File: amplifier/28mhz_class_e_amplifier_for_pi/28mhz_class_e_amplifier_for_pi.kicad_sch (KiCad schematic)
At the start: 23 parts, among them J1 Conn_Coaxial_Small, J2 694106301002, M1 RD16HHF1, U1 LT1818

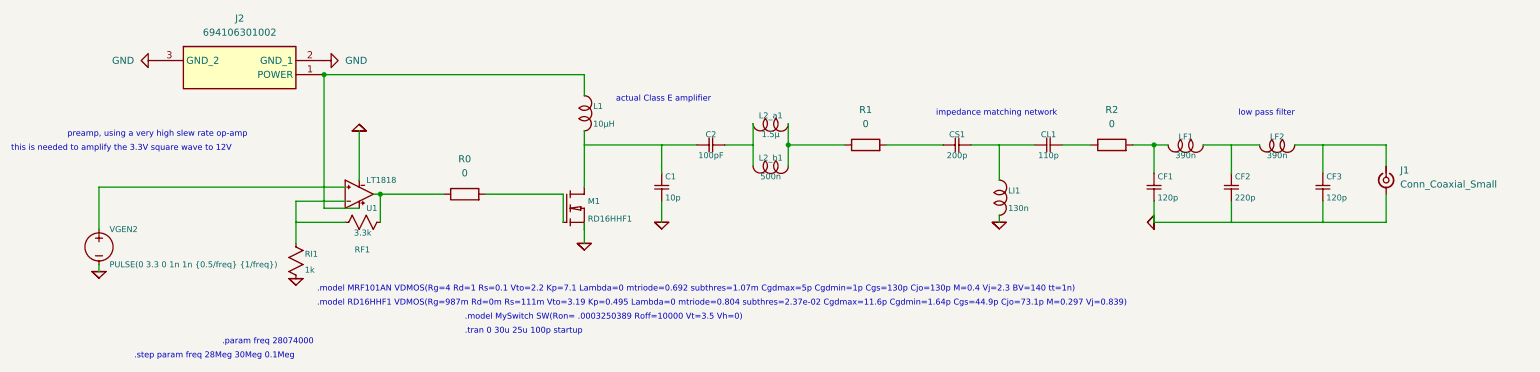
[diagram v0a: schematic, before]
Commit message: Everything except routing done
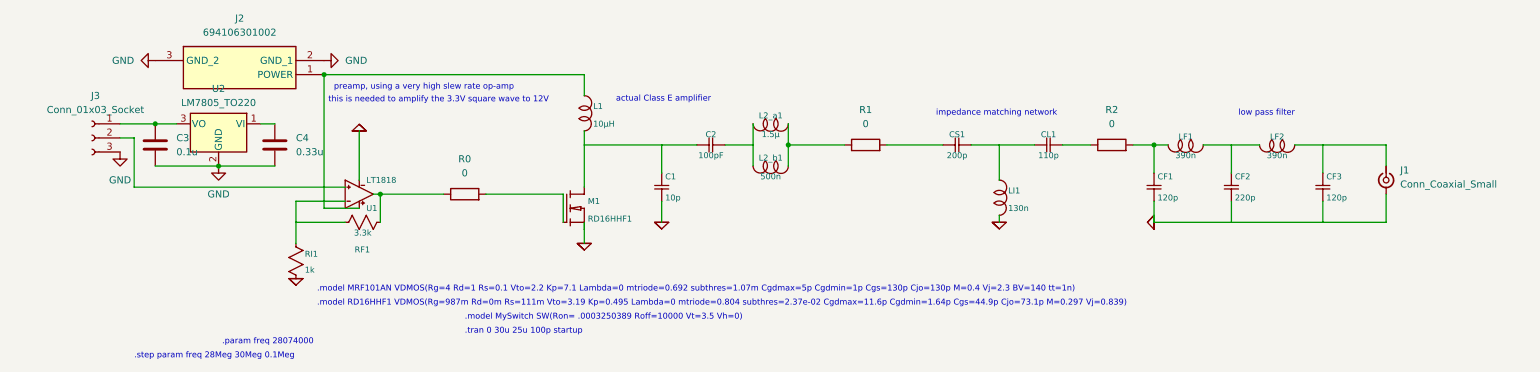
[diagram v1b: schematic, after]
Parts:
- removed VGEN2: PULSE(0 3.3 0 1n 1n {0.5/freq} {1/freq}), Connector_PinHeader_2.54mm:PinHeader_1x02_P2.54mm_Vertical, symbol ltspice:voltage
- added C3: 0.1u, Capacitor_SMD:C_0805_2012Metric, symbol Device:C
- added C4: 0.33u, Capacitor_SMD:C_0805_2012Metric, symbol Device:C
- added J3: Conn_01x03_Socket, Connector_PinSocket_2.54mm:PinSocket_1x03_P2.54mm_Vertical, symbol Connector:Conn_01x03_Socket
- added U2: LM7805_TO220, Package_TO_SOT_THT:TO-220-3_Vertical, symbol Regulator_Linear:LM7805_TO220
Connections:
- net GND: now also C3.2, C4.2, J3.3 (Pin_3), U2.2 (GND)
- net at U1.1 (IN+): now also J3.2 (Pin_2)
- new net: C3.1, J3.1 (Pin_1), U2.3 (VO)
- new net: C4.1, U2.1 (VI)
